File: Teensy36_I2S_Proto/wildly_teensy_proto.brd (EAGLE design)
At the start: 100 x 85.1 mm, 25 parts, among them CON1 MIKROE_BUS_CONN, SW2 Push_Button

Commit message: Fix/Swap RTS and CTS connections
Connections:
- net CTS_OF_GSM: now also CON1.P$15; no longer CON1.P$3, R1.2
- net RTS_OF_GSM: now also CON1.P$3, R1.2; no longer CON1.P$15
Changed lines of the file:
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@@
 <wire x1="63.5" y1="5.08" x2="43.18" y2="60.96" width="0" layer="19" extent="1-1"/>
-</signal>
-<signal name="CTS_OF_GSM">
-<contactref element="U$1" pad="33"/>
-<contactref element="CON1" pad="P$3"/>
-<contactref element="R1" pad="2"/>
-<wire x1="66.04" y1="5.08" x2="86.36" y2="60.96" width="0" layer="19" extent="1-1"/>
-<wire x1="-14.29" y1="80.01" x2="86.36" y2="60.96" width="0" layer="19" extent="1-1"/>
-</signal>
-<signal name="RTS_OF_GSM">
-<contactref element="U$1" pad="34"/>
-<contactref element="CON1" pad="P$15"/>
-<wire x1="63.5" y1="27.94" x2="83.82" y2="60.96" width="0" layer="19" extent="1-1"/>
 </signal>
 <signal name="N$2">
@@
 <wire x1="-46.67" y1="80.01" x2="73.66" y2="60.96" width="0" layer="19" extent="1-1"/>
 </signal>
-<signal name="N$22">
-</signal>
 <signal name="N$23">
 <contactref element="R9" pad="2"/>
@@
 <wire x1="-46.99" y1="61.18" x2="-44.77" y2="80.01" width="0" layer="19" extent="1-1"/>
 </signal>
+<signal name="RTS_OF_GSM">
+<contactref element="U$1" pad="34"/>
+<contactref element="CON1" pad="P$3"/>
+<contactref element="R1" pad="2"/>
+<wire x1="66.04" y1="5.08" x2="83.82" y2="60.96" width="0" layer="19" extent="1-1"/>
+<wire x1="-14.29" y1="80.01" x2="83.82" y2="60.96" width="0" layer="19" extent="1-1"/>
+</signal>
+<signal name="CTS_OF_GSM">
+<contactref element="CON1" pad="P$15"/>
+<contactref element="U$1" pad="33"/>
+<wire x1="63.5" y1="27.94" x2="86.36" y2="60.96" width="0" layer="19" extent="1-1"/>
+</signal>
 </signals>

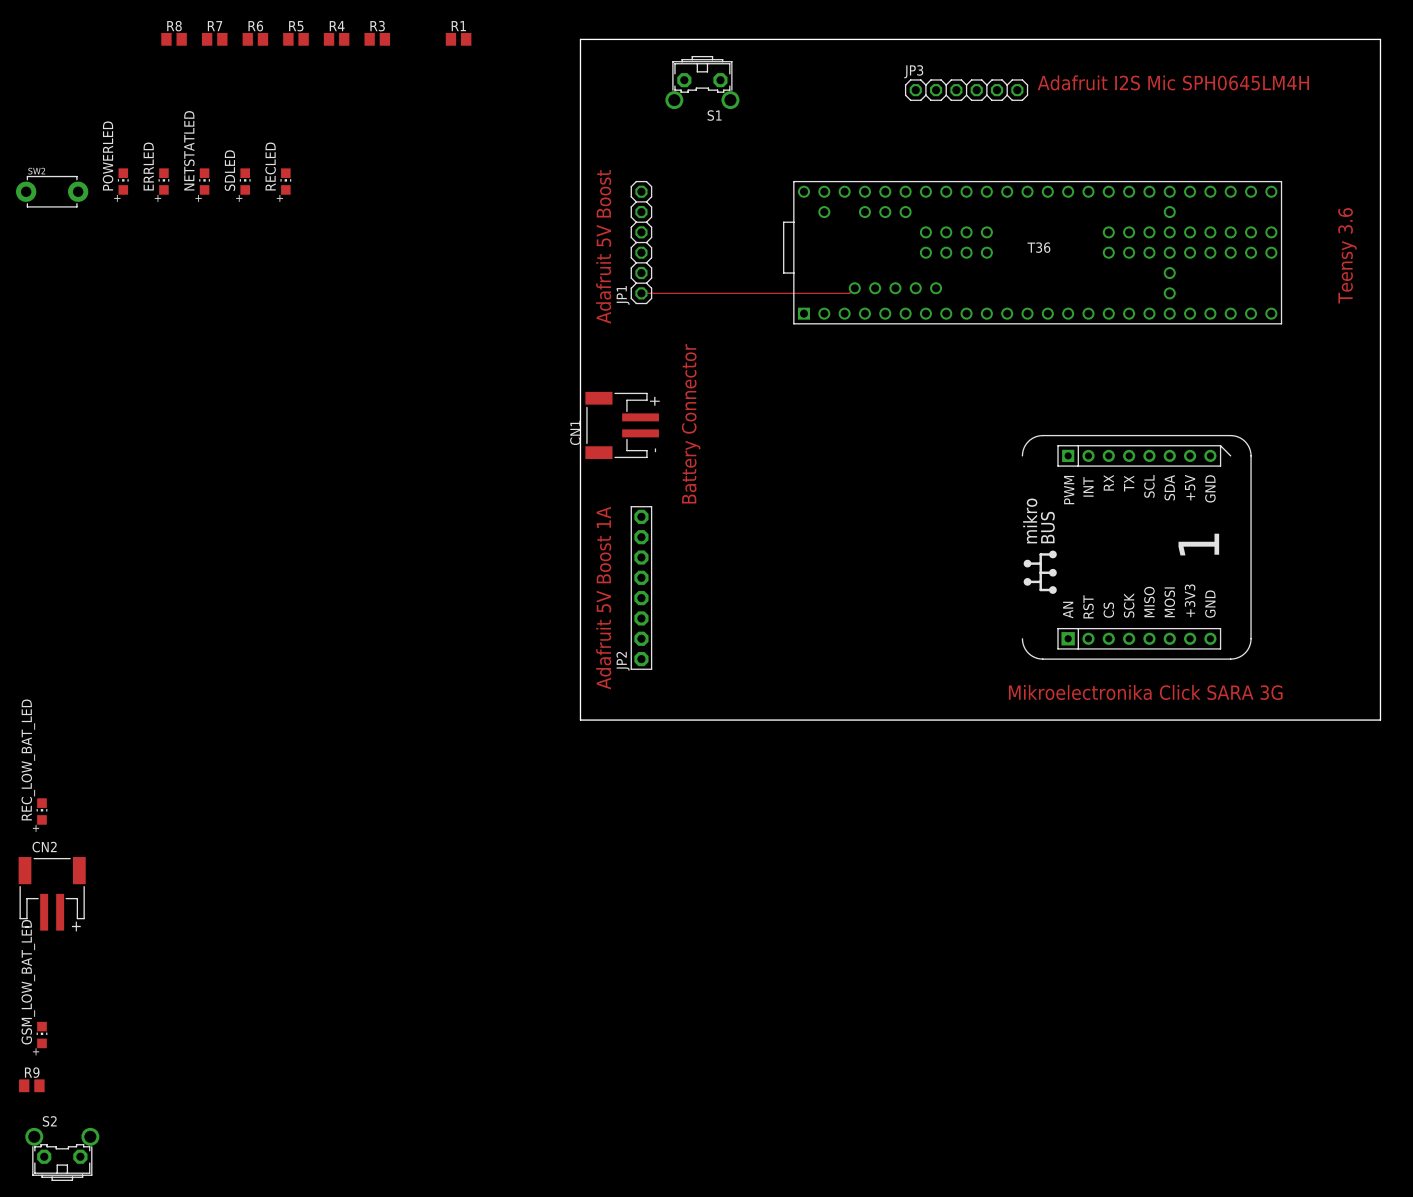
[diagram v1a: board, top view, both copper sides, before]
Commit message: Compoenent placement, Ground plane, drill holes etc on the layout
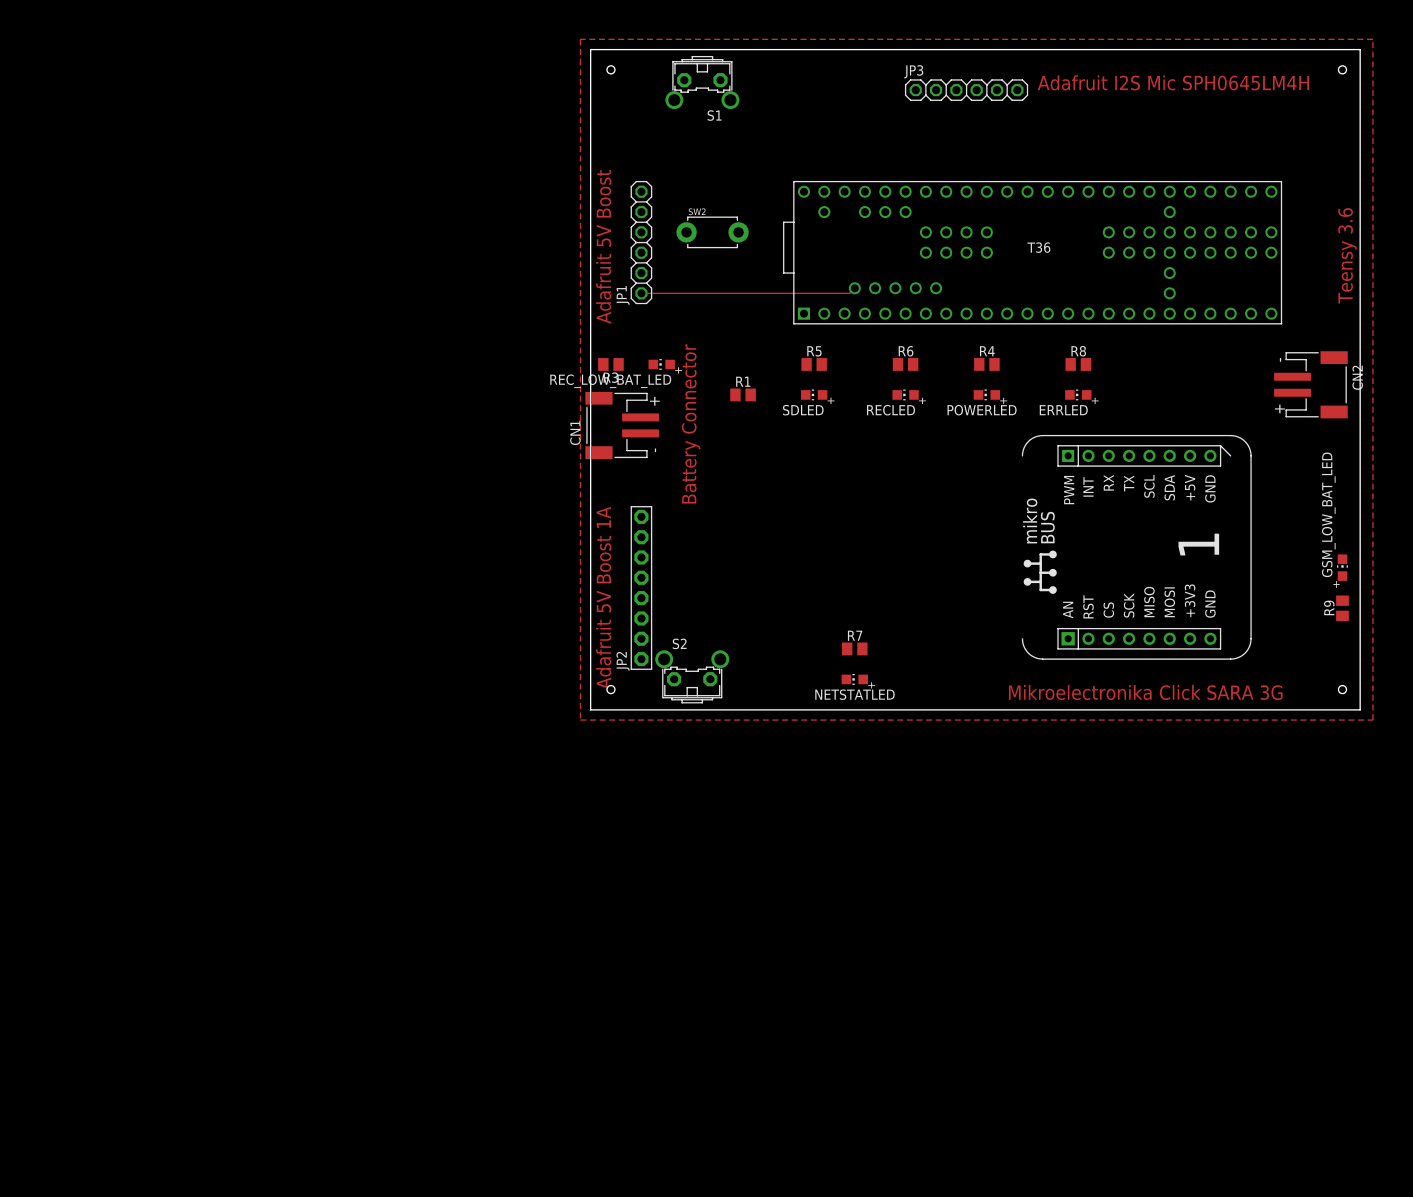
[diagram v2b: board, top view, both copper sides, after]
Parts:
- moved R9 174.4 mm to (95.2, 8.89), turned to 90 degrees
- moved GSM_LOW_BAT_LED 172.7 mm to (95.2, 14.0)
- moved CN2 170.5 mm to (92.7, 36.8), turned to 270 degrees
- moved R8 120.1 mm to (62.2, 39.4)
- moved ERRLED 117.4 mm to (62.2, 35.6), turned to 90 degrees
- moved POWERLED 111.2 mm to (50.8, 35.6), turned to 90 degrees
- moved R7 110.5 mm to (34.3, 3.81)
- moved NETSTATLED 102.4 mm to (34.3, 0.00), turned to 90 degrees
- moved S2 98.8 mm to (14.0, 1.27)
- moved REC_LOW_BAT_LED 95.5 mm to (10.2, 39.4), turned to 90 degrees
- moved R4 90.9 mm to (50.8, 39.4)
- moved R6 90.9 mm to (40.6, 39.4)
- moved SW2 82.7 mm to (16.5, 55.9)
- moved RECLED 81.9 mm to (40.6, 35.6), turned to 90 degrees
- moved R5 76.5 mm to (29.2, 39.4)
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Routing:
- added copper zone on layer 1, net GND
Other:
- board size 100 x 85.1 mm -> 96.2 x 82.5 mm

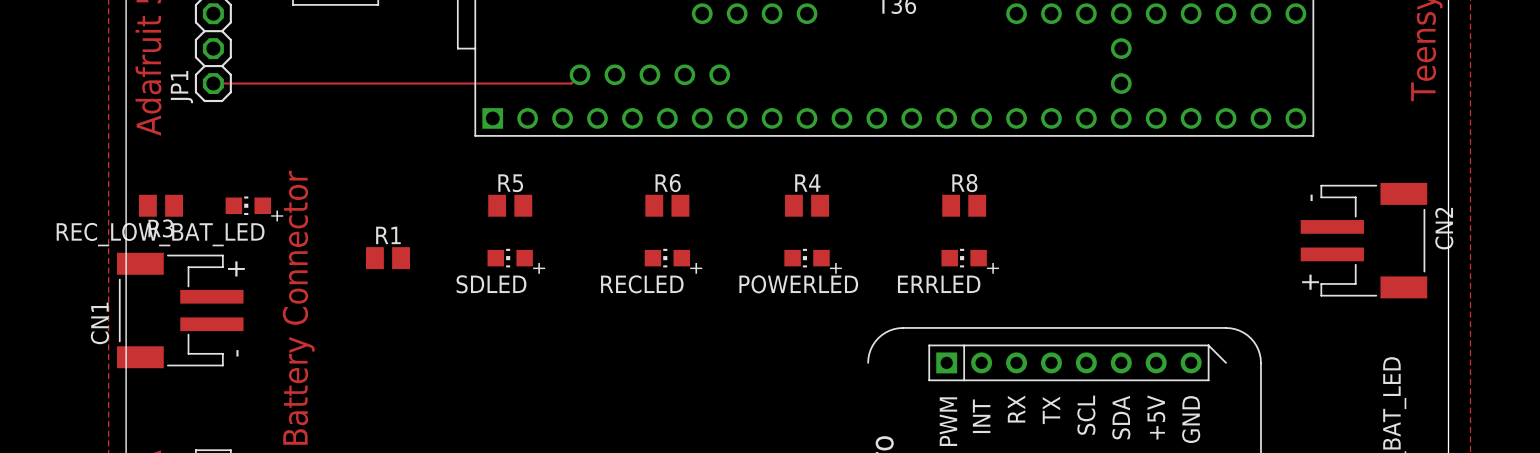
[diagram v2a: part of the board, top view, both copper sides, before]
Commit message: Clean schematics after review with Hari on 25/2/2019, BOM to be prepared
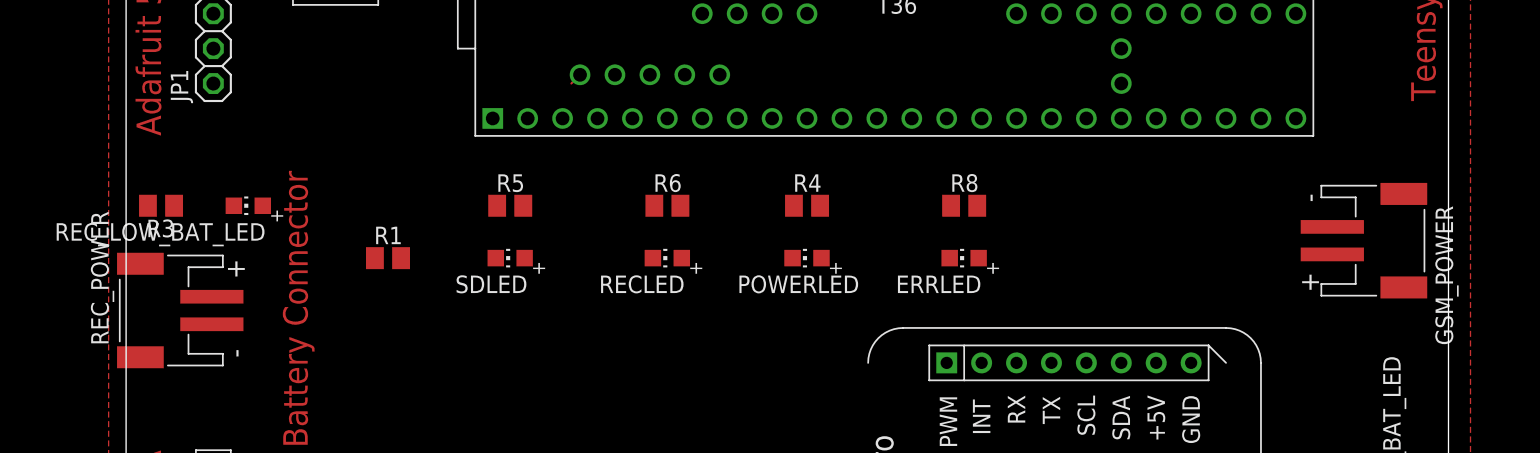
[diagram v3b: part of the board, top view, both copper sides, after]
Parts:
- R3, R4, R5, R6, R7, R8, R9: value 330R -> 1KR
- renumbered CN1 to REC_POWER, CN2 to GSM_POWER, CON1 to MIKROELECTRONIKA_SARA_CLICK
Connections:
- net 3V renamed MIC_3V
- net BCLK renamed MIC_BCLK
- net DOUT renamed MIC_DOUT
- net LRCLK renamed MIC_LRCLK
- net N$10 renamed REC_LB
- net N$2 renamed REC_5V
- net N$20 renamed GSM_LB
- net N$21 renamed NETSTATLED
- net N$24 renamed GSM_BAT
- net N$25 renamed GSM_5V
- net N$3 renamed REC_BAT
- removed net N$12: R5.1, U$1.39
- removed net N$13: R6.2, U$1.36
- removed net N$14: R8.1, U$1.37
- removed net N$15: POWERLED.A, R4.1
- removed net N$17: REC_POWER.2
- removed net N$18: JP1.5
- removed net N$19: JP2.5, S2.2
- removed net N$4: JP1.4, S1.1
- removed net N$5: R4.2, U$1.35
- new net ERRLED: R8.1, U$1.39
- new net GSM_5V_EN: JP2.5, S2.1
- new net GSM_BAT_RETURN: GSM_POWER.2, JP2.4
- new net N$3: POWERLED.A, R4.2
- new net N$6: JP2.6
- new net POWERLED: R4.1, U$1.35
- new net RECLED: R6.1, U$1.36
- new net REC_5V_EN: JP1.4, S1.2
- new net REC_BAT_RETURN: JP1.5, REC_POWER.2
- new net SDLED: R5.1, U$1.37
- net GND: now also S1.1, S2.2; no longer GSM_POWER.2, JP2.4, S1.2, S2.1
- net N$9: now also R6.2; no longer R6.1
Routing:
- net REC_5V: track 26.9 -> 0.90 mm
